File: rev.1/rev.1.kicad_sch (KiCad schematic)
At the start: 73 parts

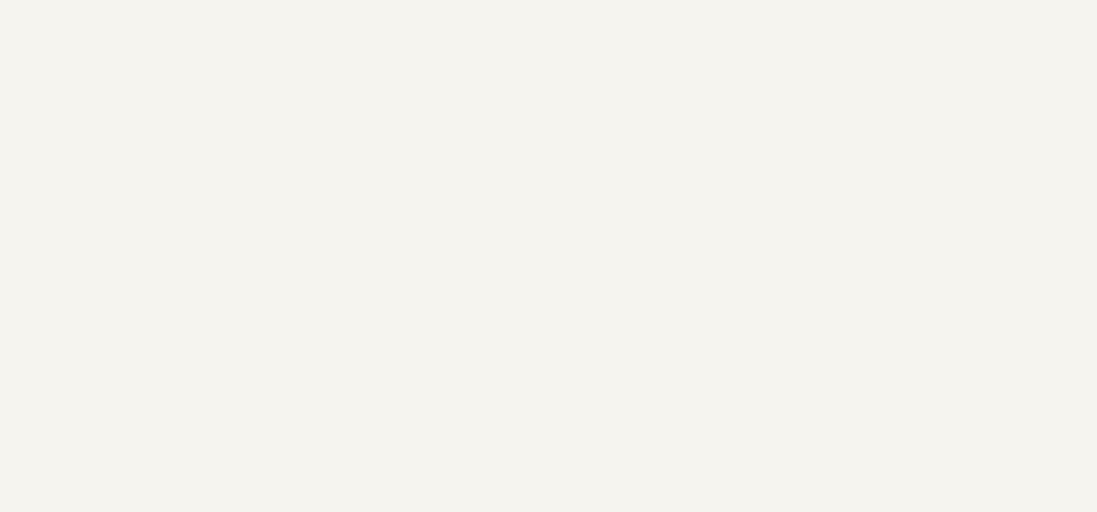
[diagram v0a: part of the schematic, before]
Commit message: добавил генератор частоты на 74ls04
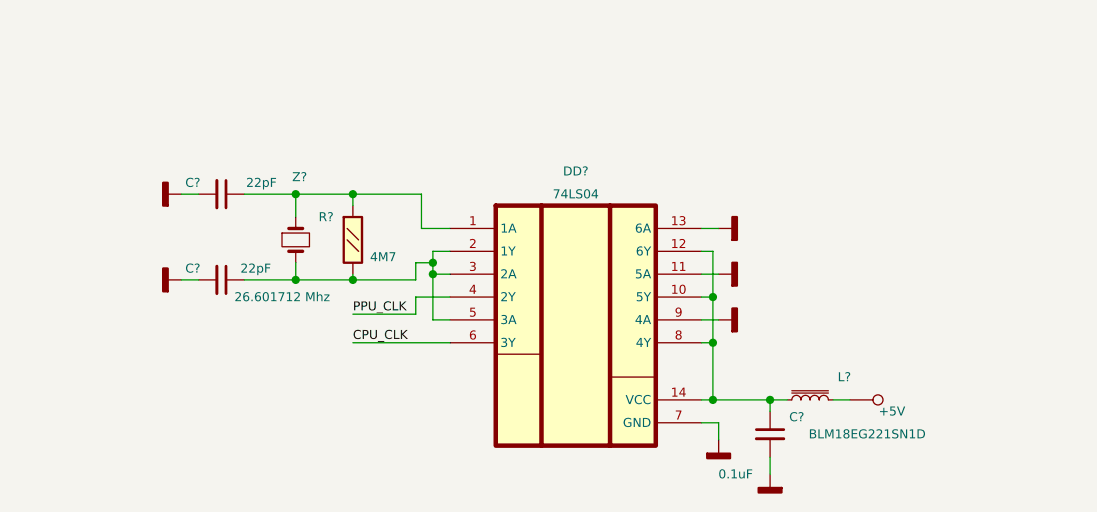
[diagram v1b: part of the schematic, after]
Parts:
- added C?: 0.1uF, symbol Device:C_Small
- added C? (x2): 22pF, symbol Device:C_Small
- added DD?: 74LS04, symbol 74xx:74HC04_gost
- added L?: BLM18EG221SN1D, symbol Device:L_Iron_Small
- added R?: 4M7, symbol Resistor_gost:R_125
- added Z?: 26.601712 Mhz, symbol Device_gost:Crystal_Small
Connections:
- net +5V: now also L?.1
- net CPU_CLK: now also DD?.6 (3Y)
- net GNDD: now also C?.2, C?.2, C?.2, DD?.11 (5A), DD?.13 (6A), DD?.7 (GND), DD?.9 (4A)
- net PPU_CLK: now also DD?.4 (2Y)
- new net: C?.1, DD?.10 (5Y), DD?.12 (6Y), DD?.14 (VCC), DD?.8 (4Y), L?.2
- new net: C?.1, DD?.1 (1A), R?.2, Z?.1
- new net: C?.1, DD?.2 (1Y), DD?.3 (2A), DD?.5 (3A), R?.1, Z?.2
